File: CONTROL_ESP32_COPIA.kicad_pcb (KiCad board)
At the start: 2 copper layers, 135.9 x 66 mm, 28 parts, among them J1 Screw_Terminal_01x02, J2 Screw_Terminal_01x04, J3 Screw_Terminal_01x04, SW1 SW_Push_SPDT, SW2 SW_Push, SW3 SW_Push, SW4 SW_Push, SW5 SW_Push, U1 ESP32-DEVKITC-32D, U2 LM7805_TO220, U3 COM-09032, U4 COM-09032

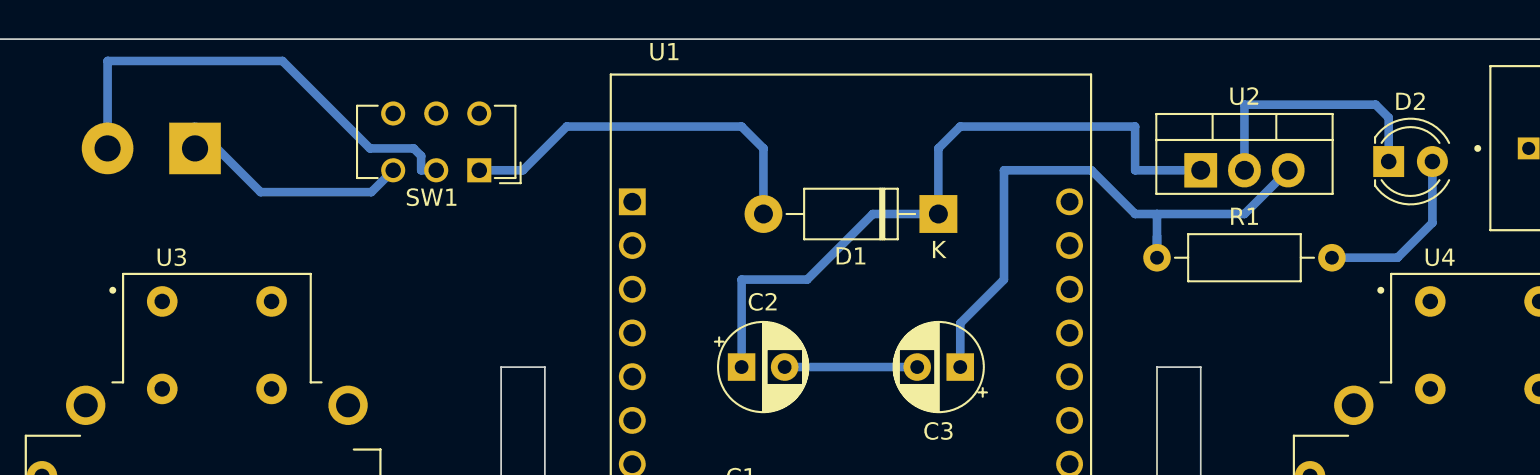
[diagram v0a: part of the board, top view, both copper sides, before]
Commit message: add copia
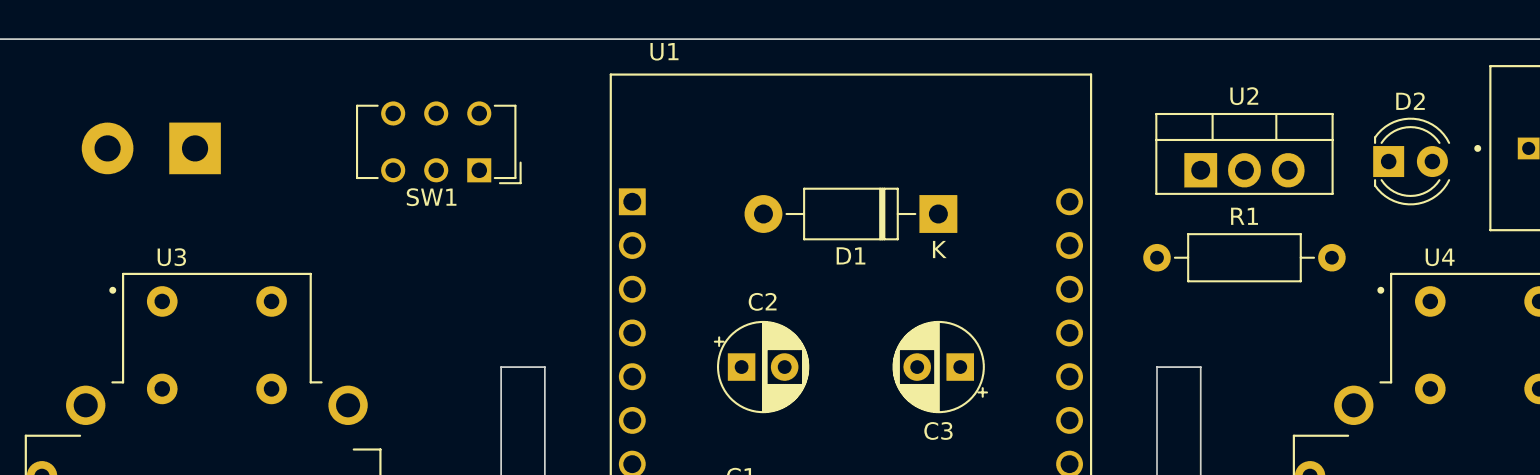
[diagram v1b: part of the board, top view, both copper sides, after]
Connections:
- net Net-(C2-Pad1) renamed VEE
- net Net-(J1-Pad2) renamed VCC
- C3 pad 1: Net-(C3-Pad1) -> +5V
- R1 pad 1: Net-(C3-Pad1) -> +5V
- U2 pad 3: Net-(C3-Pad1) -> +5V
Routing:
- net VEE: track 40.2 -> 0.00 mm
- net GND: track 36.4 -> 0.00 mm
- net Net-(C3-Pad1): track 34.9 -> 0.00 mm
- net VCC: track 26.0 -> 0.00 mm
- net Net-(D1-Pad2): track 21.9 -> 0.00 mm
- net Net-(D2-Pad2): track 10.2 -> 0.00 mm
